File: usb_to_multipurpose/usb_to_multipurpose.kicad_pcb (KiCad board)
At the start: 2 copper layers, 27 x 29 mm, 31 parts, among them U1 FT232H, U2 AP2112K-3.3TRG1, U5 93LC56BT-I/OT, Y1 12MHz

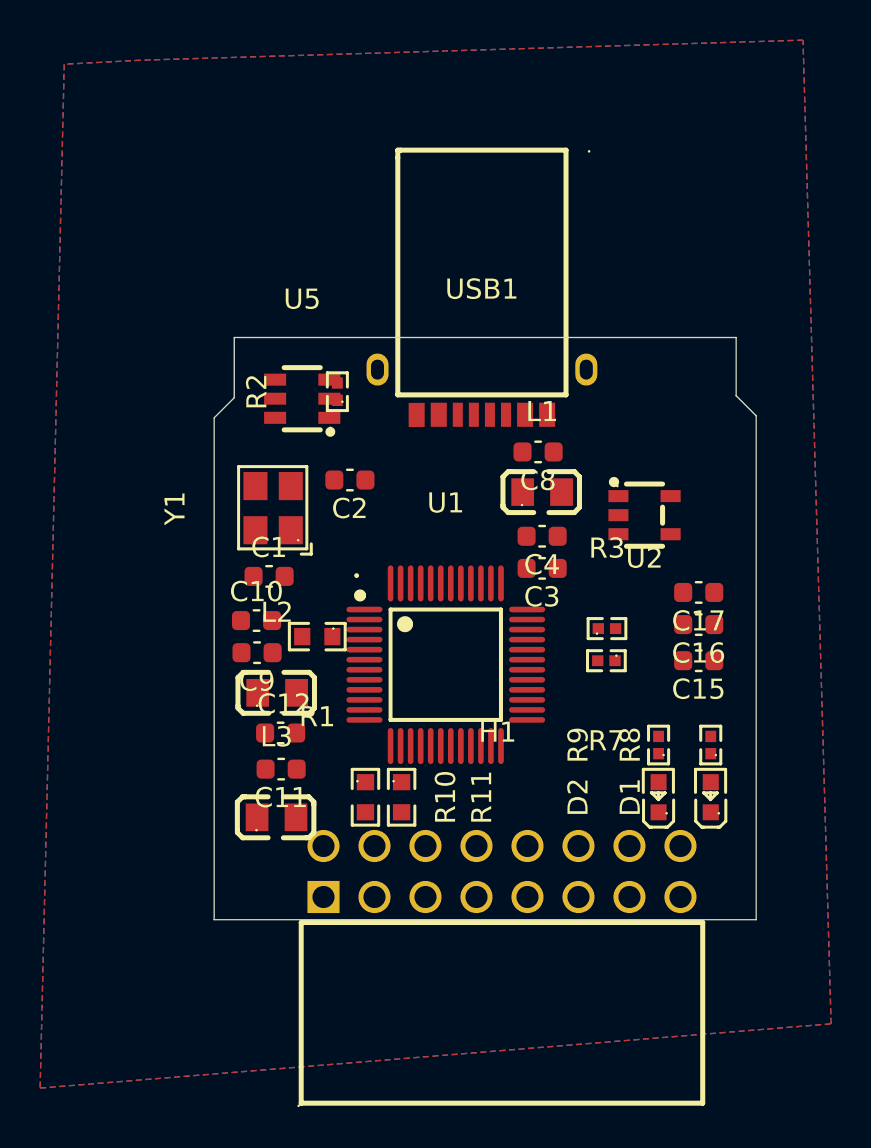
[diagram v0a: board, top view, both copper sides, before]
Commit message: Prepare v1.0 of the PCB.
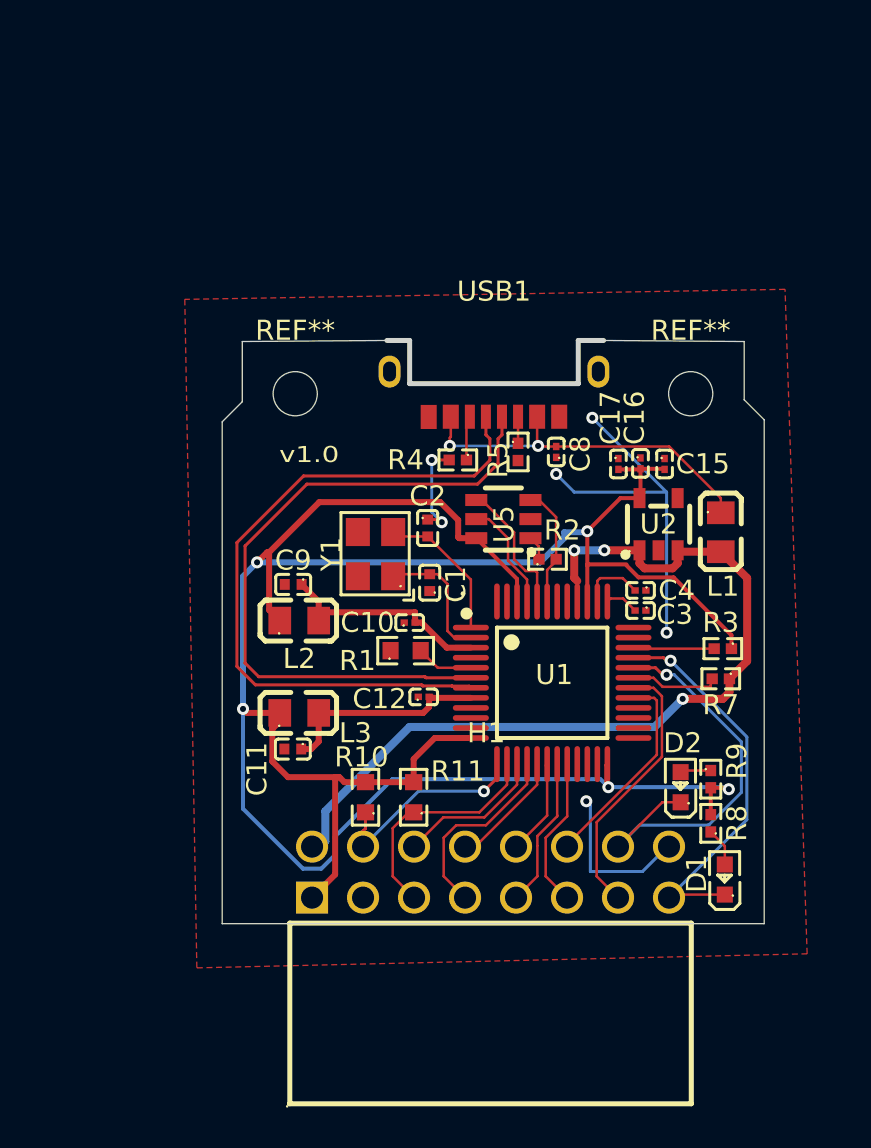
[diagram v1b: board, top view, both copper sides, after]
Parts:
- added R4: 5K1, easyeda2kicad:R0402, F.Cu at (53.4, 40.6)
- added R5: 5K1, easyeda2kicad:R0402, F.Cu at (56.4, 40.2)
- added REF**: MountingHole_2.2mm_M2, MountingHole:MountingHole_2.2mm_M2, F.Cu at (65.0, 37.3)
- added REF**: MountingHole_2.2mm_M2, MountingHole:MountingHole_2.2mm_M2, F.Cu at (45.3, 37.3)
- C1, C11, C2, C9: footprint Capacitor_SMD:C_0603_1608Metric -> easyeda2kicad:C0402
- C10, C12, C15, C16, C17, C3, C4, C8: footprint Capacitor_SMD:C_0603_1608Metric -> easyeda2kicad:C0201
- moved R2 13.4 mm to (57.9, 45.5), turned to 0 degrees
- moved U5 11.7 mm to (55.7, 43.5)
- moved C15 9.95 mm to (63.7, 40.8), turned to -90 degrees
- moved L1 9.12 mm to (66.5, 44.2), turned to -90 degrees
- moved C16 8.54 mm to (62.5, 40.8), turned to -90 degrees
- moved C1 8.01 mm to (52.0, 46.7), turned to 90 degrees
- moved C10 7.63 mm to (51.0, 48.7)
- moved C17 7.55 mm to (61.4, 40.8), turned to -90 degrees
- moved C12 7.35 mm to (51.7, 52.4)
- moved R3 5.86 mm to (66.6, 50.0), turned to 180 degrees
- moved R7 5.77 mm to (66.5, 51.5)
- moved C4 5.59 mm to (62.5, 47.1)
- moved Y1 5.59 mm to (49.3, 45.3)
- moved U1 5.38 mm to (58.1, 51.7)
- moved C3 5.33 mm to (62.5, 48.1)
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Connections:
- H1 pad 10: Net-(U1-ADBUS6) -> Net-(U1-ADBUS5)
- H1 pad 9: Net-(U1-ADBUS5) -> Net-(U1-ADBUS6)
- USB1 pad 1: unconnected-(USB1-SHELL-Pad1) -> GND
- USB1 pad 2: unconnected-(USB1-SHELL-Pad2) -> GND
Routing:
- net VCC: track 0.00 -> 125.7 mm, vias 0 -> 5
- net +5V: track 0.00 -> 43.6 mm, vias 0 -> 3
- net /D+: track 0.00 -> 34.8 mm
- net /D-: track 0.00 -> 34.1 mm
- net GND: track 0.00 -> 31.1 mm, vias 0 -> 6
- net Net-(D2-K): track 0.00 -> 20.7 mm, vias 0 -> 1
- net Net-(D1-K): track 0.00 -> 19.7 mm, vias 0 -> 1
- net Net-(C8-Pad2): track 0.00 -> 18.3 mm, vias 0 -> 2
- net Net-(U1-ACBUS6): track 0.00 -> 13.4 mm
- net /SDA/MOSI: track 0.00 -> 11.5 mm
- net /VPHY: track 0.00 -> 10.9 mm
- net /VPLL: track 0.00 -> 10.7 mm
- net /SCL/SCK: track 0.00 -> 10.5 mm, vias 0 -> 1
- net Net-(U1-ACBUS5): track 0.00 -> 10.4 mm
- net /CS: track 0.00 -> 9.68 mm
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- removed copper zone on B.Cu, net GND
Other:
- board size 27 x 29 mm -> 27 x 29.1 mm
- board text added: "v1.0"
